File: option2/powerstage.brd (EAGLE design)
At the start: 42 x 43.5 mm, 40 parts, among them CON1 PINHEAD_1X10-2-FEMALE, CON2 BATTERY_CON-2P-XT30-RA, CON3 PINHEAD_1X10-2-FEMALE, IC5 MCP9700, Q1 BUK7K6R2-40EX, Q2 BUK7K6R2-40EX, Q3 BUK7K6R2-40EX

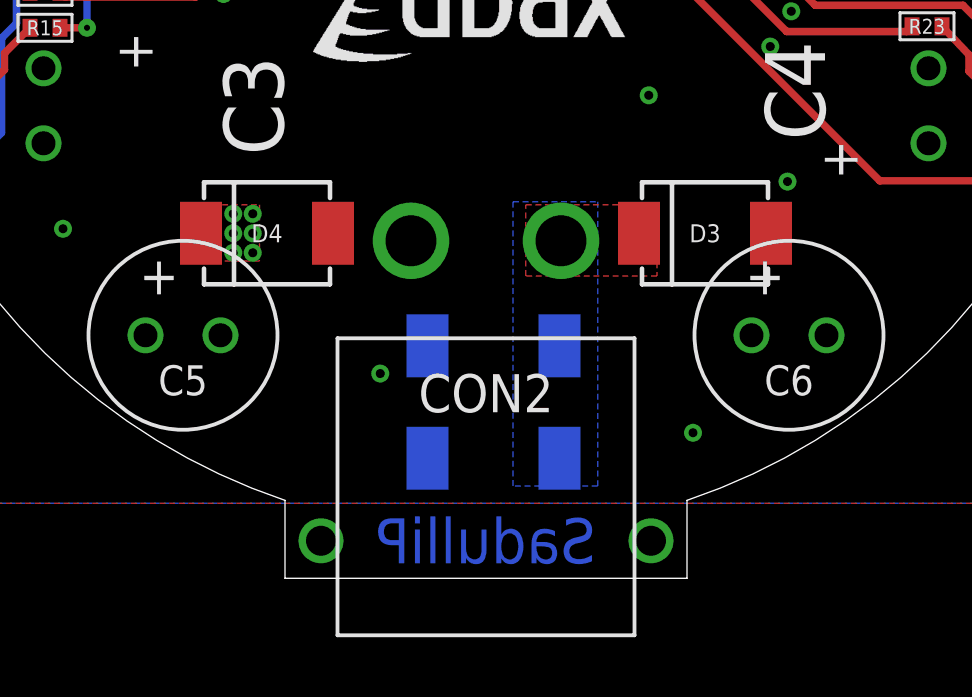
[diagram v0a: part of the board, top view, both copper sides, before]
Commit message: updates here and there
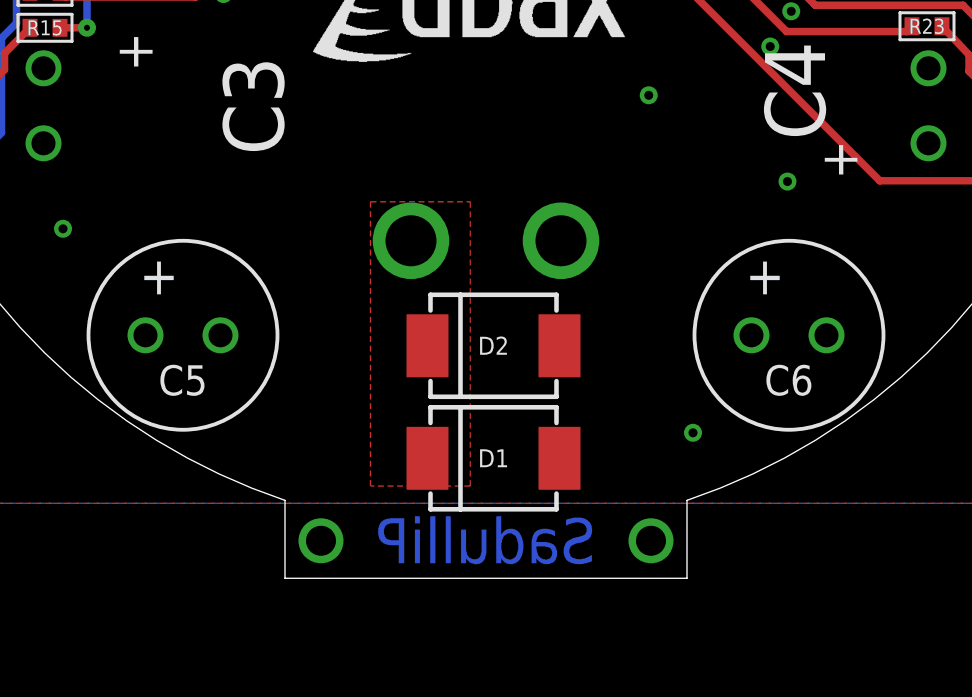
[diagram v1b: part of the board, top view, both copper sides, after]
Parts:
- removed D3, D4: PTVS36VP1UP,115-36V-SOD128, TVS_diodes:SOD128
- flipped CON2 to the bottom
- flipped D1 to the top
- flipped D2 to the top
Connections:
- net PGND: no longer D3.A, D4.A
- net VDC: no longer D3.C, D4.C
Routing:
- net VDC: track 0.80 -> 0.22 mm, vias 57 -> 51
